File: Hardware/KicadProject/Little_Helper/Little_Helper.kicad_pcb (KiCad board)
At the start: 4 copper layers, 84 x 19.6 mm, 15 parts, among them J2 USB_C_Receptacle_USB2.0_16P, SW1 SW_Push, SW2 SW_Push, SW3 SW_Push, SW4 SW_Push, SW5 SW_Push, U1 ESP32-S3-MINI-1

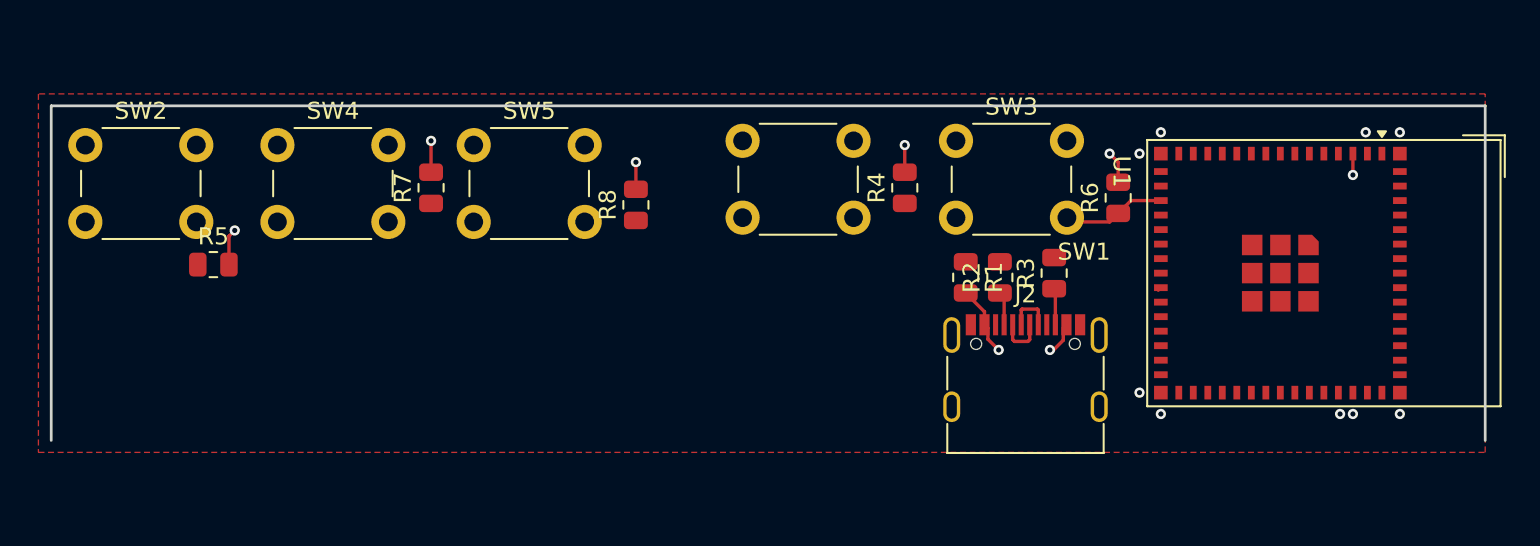
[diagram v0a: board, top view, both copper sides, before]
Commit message: board in progress
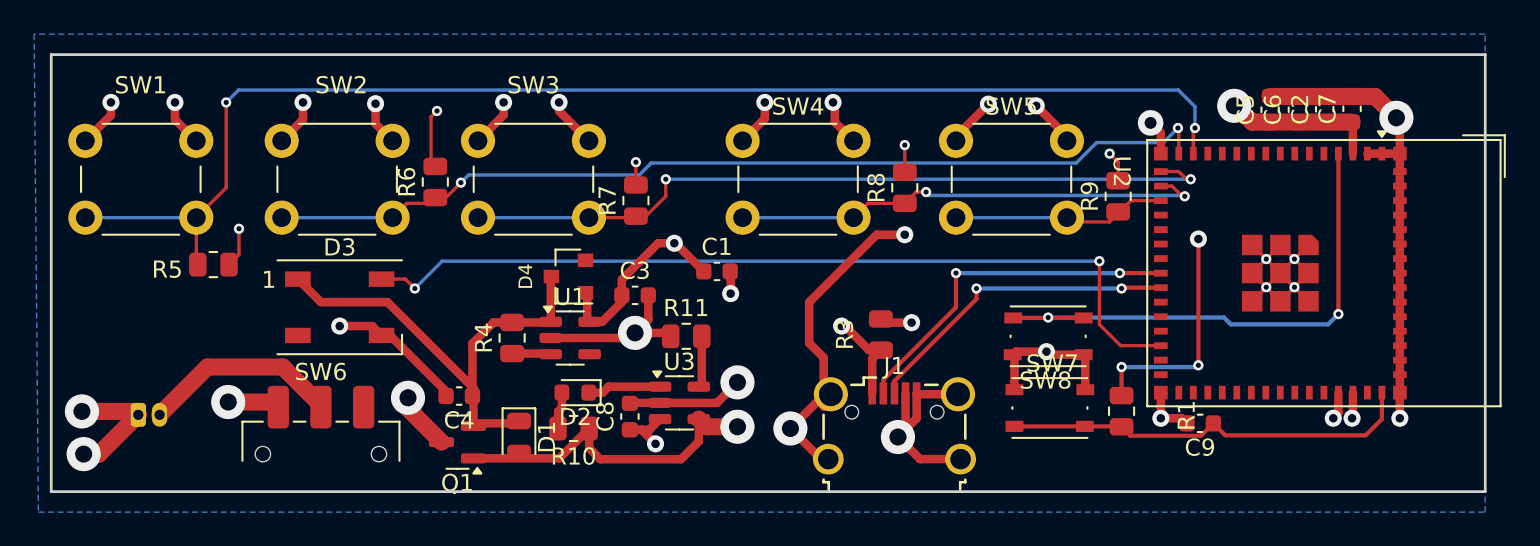
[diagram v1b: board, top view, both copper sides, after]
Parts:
- removed the R3 at (16.8, 0.00)
- added C1: 10uF, Capacitor_SMD:C_0603_1608Metric, F.Cu at (-3.00, -0.10)
- added C2: 10uF, Capacitor_SMD:C_0603_1608Metric, F.Cu at (32.6, -9.60)
- added C3: 10uF, Capacitor_SMD:C_0603_1608Metric, F.Cu at (-7.80, 1.30)
- added C4: 10uF, Capacitor_SMD:C_0603_1608Metric, F.Cu at (-18.1, 7.20)
- added C5: 10uF, Capacitor_SMD:C_0603_1608Metric, F.Cu at (29.4, -9.57)
- added C6: 10uF, Capacitor_SMD:C_0603_1608Metric, F.Cu at (31.0, -9.57)
- added C7: 1uF, Capacitor_SMD:C_0603_1608Metric, F.Cu at (34.2, -9.62)
- added C8: 10uF, Capacitor_SMD:C_0603_1608Metric, F.Cu at (-8.10, 8.40)
- added C9: 1uF, Capacitor_SMD:C_0603_1608Metric, F.Cu at (25.3, 8.80)
- added D1: MBR0540, Diode_SMD:D_0805_2012Metric, F.Cu at (-14.6, 9.60)
- added D2: LED, LED_SMD:LED_0603_1608Metric, F.Cu at (-11.3, 7.00)
- added D3: WS2812B, LED_SMD:LED_WS2812B_PLCC4_5.0x5.0mm_P3.2mm, F.Cu at (-25.1, 2.00)
- added D4: BAS16, ba_sot:sot_23, F.Cu at (-11.7, 0.20)
- added J2: Conn_01x02_Pin, Connector_Hirose:Hirose_DF13-02P-1.25DSA_1x02_P1.25mm_Vertical, B.Cu at (-36.9, 8.30)
- added Q1: DMG3415U, Package_TO_SOT_SMD:SOT-23, F.Cu at (-18.2, 9.90)
- added R10: 5k1, Resistor_SMD:R_0805_2012Metric, F.Cu at (-11.4, 9.10)
- added R11: 5k1, Resistor_SMD:R_0805_2012Metric, F.Cu at (-4.80, 3.70)
- added R9: 10k, Resistor_SMD:R_0805_2012Metric, F.Cu at (20.5, -4.50)
- added SW6: SW_SPST, Button_Switch_SMD:SW_SPDT_CK_JS102011SAQN, F.Cu at (-26.2, 10.6)
- added SW7: SW_Push, Button_Switch_SMD:SW_Push_1P1T_NO_Vertical_Wuerth_434133025816, F.Cu at (16.5, 7.90)
- added SW8: SW_Push, Button_Switch_SMD:SW_Push_1P1T_NO_Vertical_Wuerth_434133025816, F.Cu at (16.4, 3.70)
- added U1: AP2112K-3.3, Package_TO_SOT_SMD:SOT-23-5, F.Cu at (-11.6, 3.80)
- added U3: MCP73831-2-OT, Package_TO_SOT_SMD:SOT-23-5, F.Cu at (-5.20, 7.60)
- J1: renamed from J2; value USB_C_Receptacle_USB2.0_16P -> USB_B_Micro; footprint Connector_USB:USB_C_Receptacle_G-Switch_GT-USB-7010ASV -> Connector_USB:USB_Micro-B_Wuerth_629105150521_CircularHoles
- R3: renamed from R1; value 100k -> R2012_100K; footprint Resistor_SMD:R_0805_2012Metric -> ba_res:r2012
- R4: value 10k -> 100k
- moved SW1 45.2 mm to (-40.0, -7.75), turned to 0 degrees
- moved R6 40.0 mm to (-19.5, -5.34)
- moved SW5 28.3 mm to (11.0, -7.75)
- moved SW3 28.0 mm to (-17.0, -7.75)
- moved SW4 27.3 mm to (-1.50, -7.75)
- moved R4 24.6 mm to (-15.0, 3.80)
- moved R8 15.8 mm to (8.00, -5.00)
- moved R7 12.0 mm to (-7.75, -4.25)
- moved SW2 11.5 mm to (-28.5, -7.75)
- moved R1 10.6 mm to (20.7, 8.09), turned to -90 degrees
- moved J1 7.98 mm to (7.39, 8.95)
- moved R3 5.99 mm to (6.60, 3.60), turned to 90 degrees
- renumbered R2 to R1, U1 to U2
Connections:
- R1 pad 1: Net-(J2-CC1) -> +3.3V
- R1 pad 2: GND -> /RESET
- R3 pad 1: GND -> VBUS
- R3 pad 2: VBUS -> GND
- R4 pad 1: /BTN_1_REC -> Net-(U1-EN)
- R4 pad 2: +3.3V -> /NEOPIX_VDD
- R6 pad 1: /BTN_1_PL -> /BTN_1_STOP
- R7 pad 1: /BTN_1_STOP -> /BTN_1_VW
- R8 pad 1: /BTN_1_VW -> /BTN_1_REC
- SW1 pad 2: /BTN_1_REC -> /BTN_1_RV
- SW2 pad 2: /BTN_1_RV -> /BTN_1_STOP
- SW3 pad 2: /BTN_1_PL -> /BTN_1_VW
- SW4 pad 2: /BTN_1_STOP -> /BTN_1_REC
- SW5 pad 2: /BTN_1_VW -> /BTN_1_PL
- U2 pad 28: unconnected-(U1-IO33-Pad28) -> /NEOPIX
- U2 pad 4: unconnected-(U1-IO0-Pad4) -> /BOOT0
- U2 pad 45: unconnected-(U1-EN-Pad45) -> /RESET
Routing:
- net GND: track 0.00 -> 158.8 mm, vias 9 -> 31
- net /BTN_1_RV: track 0.00 -> 76.9 mm, vias 0 -> 2
- net /BTN_1_STOP: track 0.00 -> 56.4 mm, vias 0 -> 2
- net /NEOPIX: track 0.00 -> 50.8 mm, vias 0 -> 2
- net /BTN_1_VW: track 0.00 -> 45.1 mm, vias 0 -> 2
- net +3.3V: track 10.3 -> 45.8 mm, vias 6 -> 10
- net /BOOT0: track 0.00 -> 31.0 mm, vias 0 -> 2
- net /NEOPIX_VDD: track 0.00 -> 28.8 mm
- net /BTN_1_REC: track 0.00 -> 28.3 mm, vias 0 -> 2
- net /RESET: track 0.00 -> 24.3 mm
- net VBUS: track 6.14 -> 25.2 mm
- net /Usb_D-: track 2.83 -> 20.8 mm, vias 0 -> 2
- net /Usb_D+: track 2.99 -> 19.0 mm, vias 0 -> 2
- net Net-(J2-Pin_2): track 0.00 -> 11.7 mm
- net +BATT: track 0.00 -> 9.66 mm, vias 0 -> 3
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- added copper zone on In2.Cu, net +BATT
- added copper zone on B.Cu, net GND
- removed copper zone on F.Cu, net GND
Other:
- board size 84 x 19.6 mm -> 84 x 25.6 mm
- rule pad_to_mask_clearance: 0 -> 0.05
